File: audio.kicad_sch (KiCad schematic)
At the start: 14 parts, among them J10 Audio IN Left, J11 Audio OUT Right, J12 Audio OUT Left, J8 HiFi Berry, J9 Audio IN Right

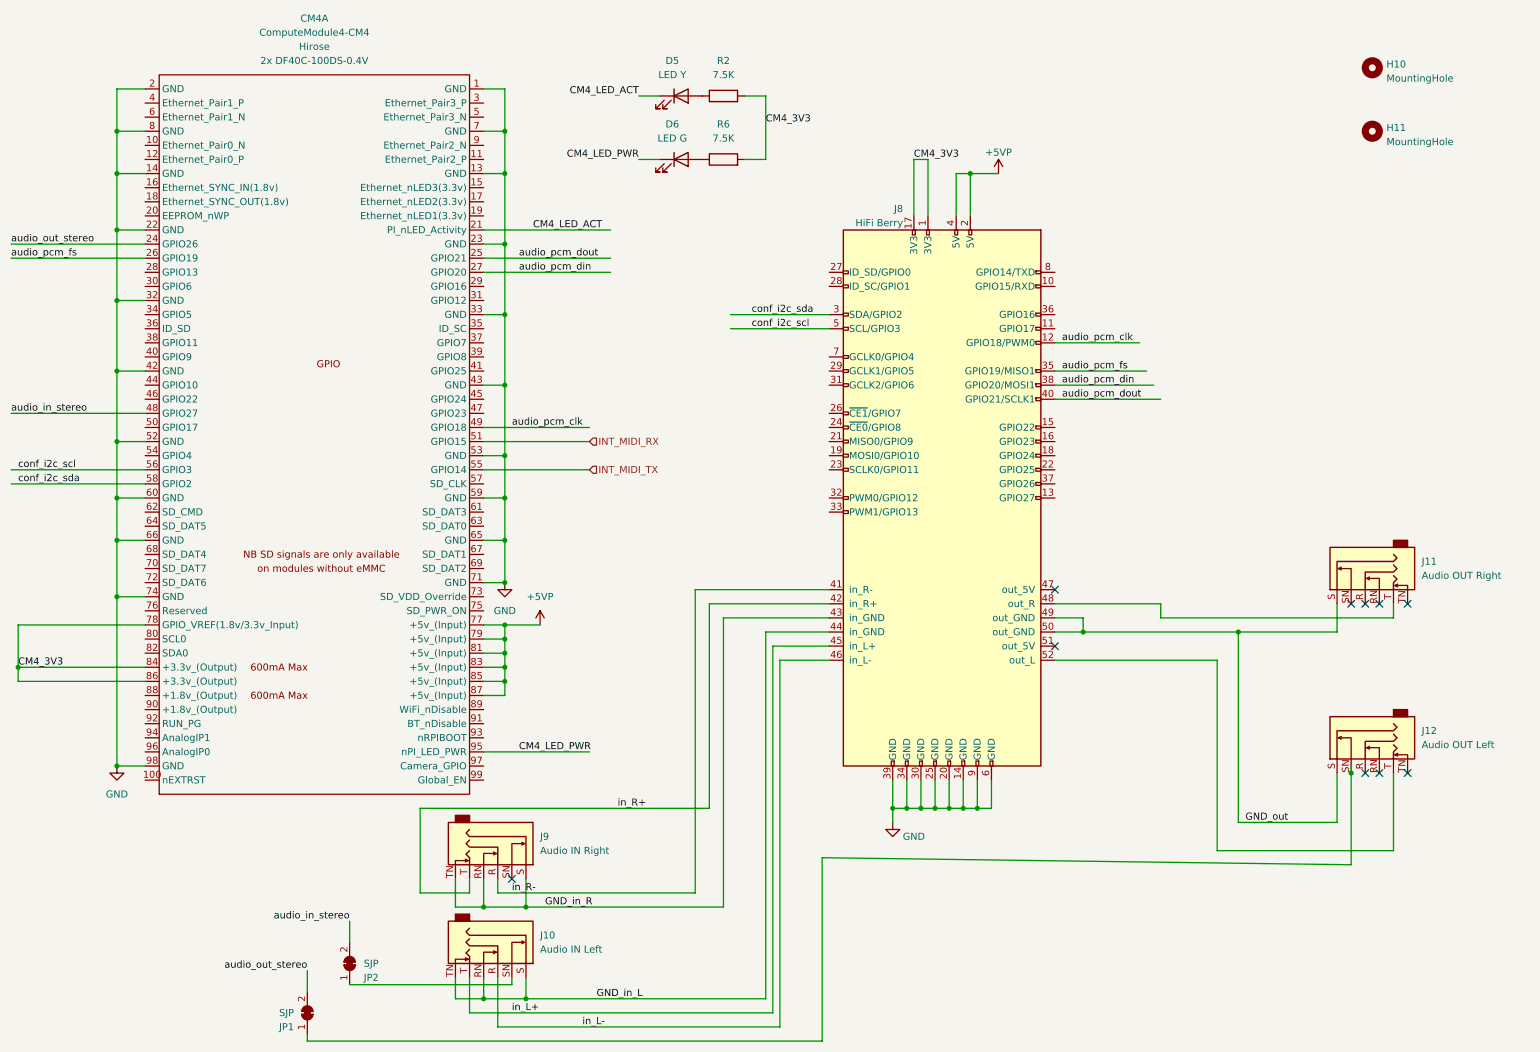
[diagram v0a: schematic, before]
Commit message: Driver for LED
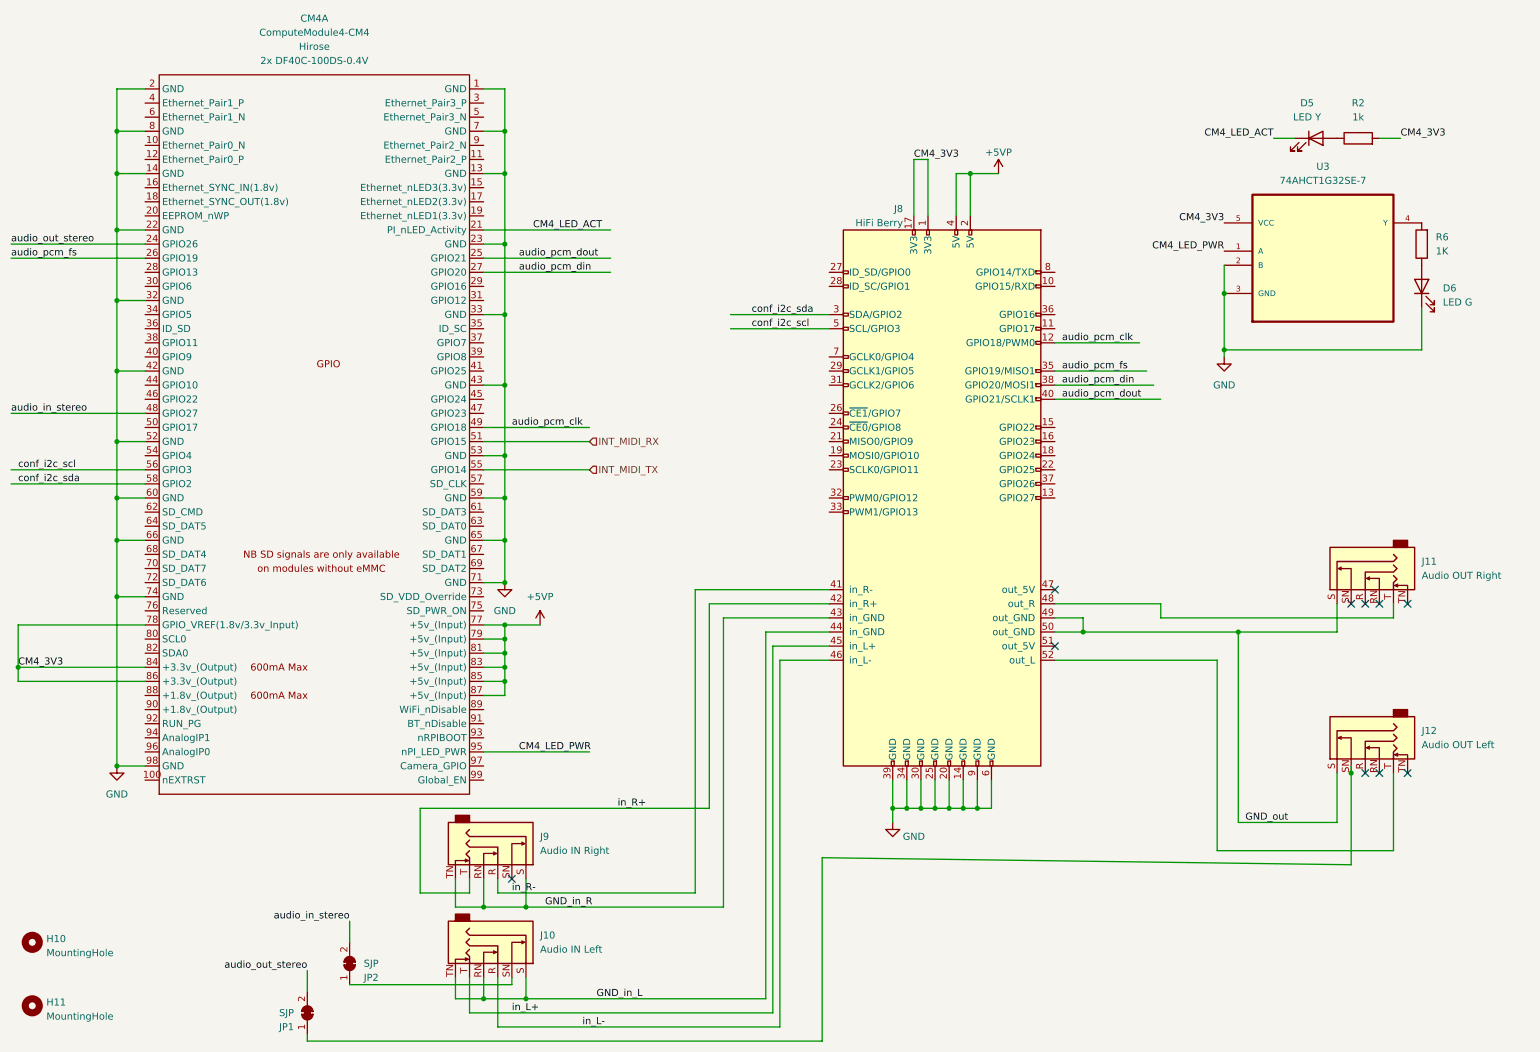
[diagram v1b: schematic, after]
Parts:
- added U3: 74AHCT1G32SE-7, SOT-353_SC-70-5, symbol 74AHCT1G32SE-7:74AHCT1G32SE-7
- R2: value 7.5K -> 1k
- R6: value 7.5K -> 1K
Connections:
- net CM4_3V3: now also U3.5 (VCC); no longer R6.2
- net CM4_LED_PWR: now also U3.1 (A); no longer D6.1 (K)
- net GND: now also D6.1 (K), U3.2 (B), U3.3 (GND)
- new net: R6.2, U3.4 (Y)
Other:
- moved on the sheet: D5, H10, H11, R2
